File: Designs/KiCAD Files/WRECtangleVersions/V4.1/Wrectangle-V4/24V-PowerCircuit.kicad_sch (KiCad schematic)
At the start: 26 parts, among them M1-24V1 60V, M2-24V1 40V, U7 TPS43060RTER

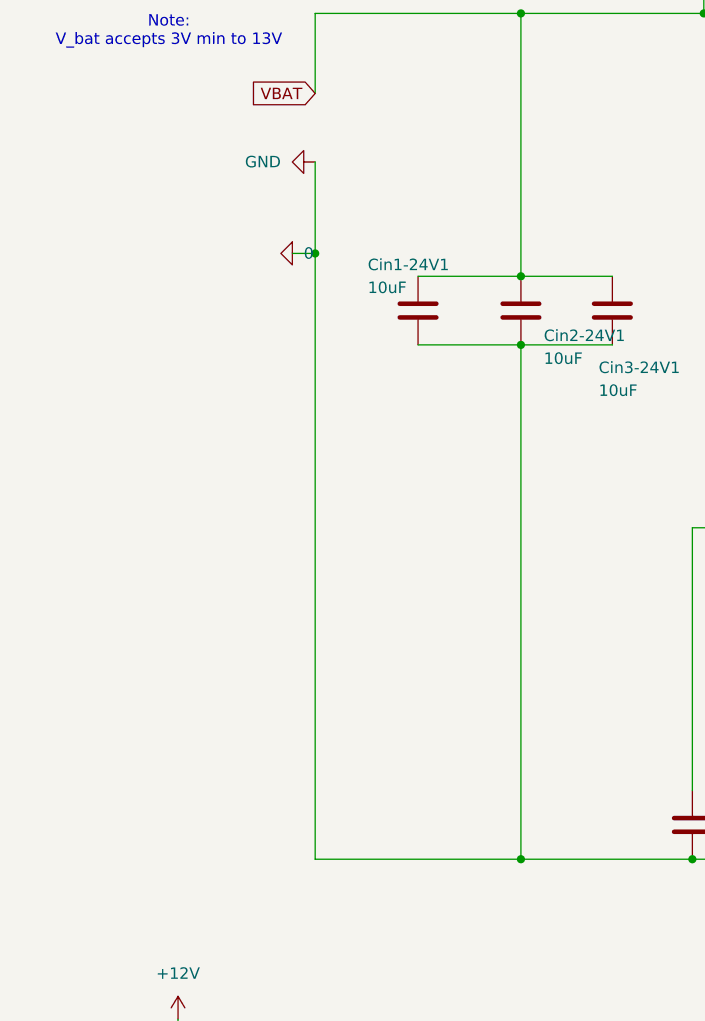
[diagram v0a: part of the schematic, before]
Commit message: all but one ERC error????
MAYBE??
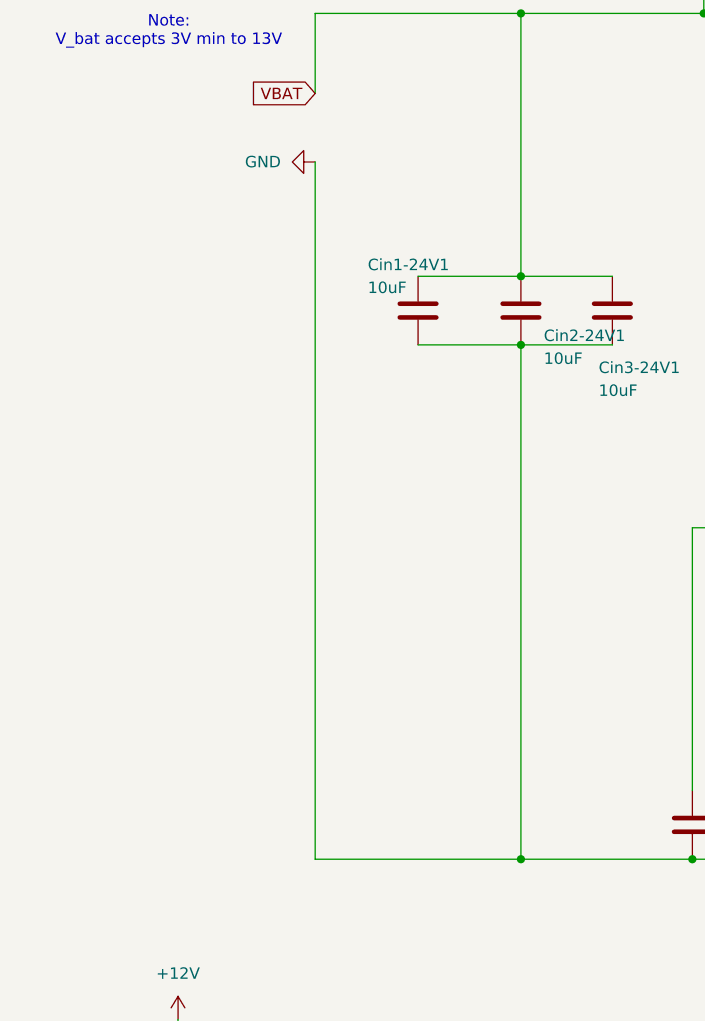
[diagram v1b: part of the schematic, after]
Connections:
- net 0 renamed GND
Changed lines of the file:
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@@
-	)
-	(junction
-		(at 53.34 72.39)
-		(diameter 0)
-		(color 0 0 0 0)
 	)
 	(junction
@@
 	(wire
 		(pts
-			(xy 50.8 72.39) (xy 53.34 72.39)
-		)
-		(stroke
-			(width 0)
-			(type default)
-		)
-	)
-	(wire
-		(pts
 			(xy 53.34 139.7) (xy 76.2 139.7)
 		)
@@
 	(wire
 		(pts
-			(xy 53.34 72.39) (xy 53.34 62.23)
+			(xy 53.34 62.23) (xy 53.34 139.7)
 		)
 		(stroke
@@
 		(pts
 			(xy 255.27 45.72) (xy 236.22 45.72)
-		)
-		(stroke
-			(width 0)
-			(type default)
-		)
-	)
-	(wire
-		(pts
-			(xy 53.34 139.7) (xy 53.34 72.39)
 		)
 		(stroke
@@
 					(unit 1)
 				)
-			)
-		)
-	)
-	(symbol
-		(lib_id "Simulation_SPICE:0")
-		(at 50.8 72.39 270)
-		(unit 1)
-		(exclude_from_sim no)
-		(in_bom yes)
-		(on_board yes)
-		(dnp no)
-		(fields_autoplaced yes)
-		(property "Reference" "#GND01"
-			(at 45.72 72.39 0)
-			(effects
-				(font
-					(size 1.27 1.27)
-				)
-				(hide yes)
-			)
-		)
-		(property "Value" "0"
-			(at 52.07 72.3899 90)
-			(effects
-				(font
-					(size 1.27 1.27)
-				)
-				(justify left)
-			)
-		)
-		(property "Footprint" ""
-			(at 50.8 72.39 0)
-			(effects
-				(font
-					(size 1.27 1.27)
-				)
-				(hide yes)
-			)
-		)
-		(property "Datasheet" "https://ngspice.sourceforge.io/docs/ngspice-html-manual/manual.xhtml#subsec_Circuit_elements__device"
-			(at 40.64 72.39 0)
-			(effects
-				(font
-					(size 1.27 1.27)
-				)
-				(hide yes)
-			)
-		)
-		(property "Description" "0V reference potential for simulation"
-			(at 43.18 72.39 0)
-			(effects
-				(font
-					(size 1.27 1.27)
-				)
-				(hide yes)
-			)
-		)
-		(pin "1"
-		)
-		(instances
-			(project ""
-				(path "/999a87cf-6a03-4be4-a445-b5341a1dddf0/a54ed999-f025-4f35-b083-b61c3d192ac9"
-					(reference "#GND01")
-					(unit 1)
-				)
